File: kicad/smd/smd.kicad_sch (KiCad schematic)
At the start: 13 parts, among them J1 Conn_01x14, J2 Conn_01x14_Socket, J4 Conn_01x03_Socket, J5 Conn_01x06, J6 Conn_01x08, J7 Conn_01x07, J8 Conn_01x09

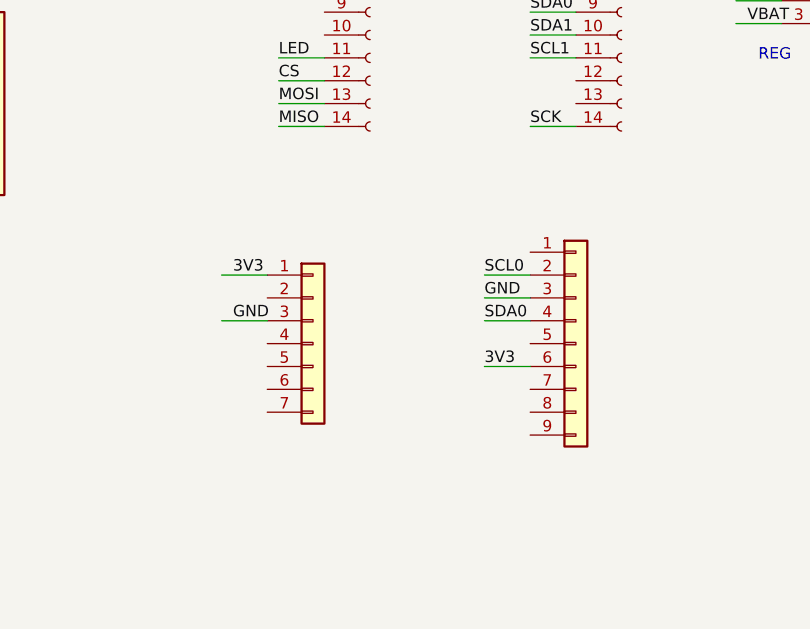
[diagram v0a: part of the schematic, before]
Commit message: modified:   kicad/smd/smd.kicad_pcb
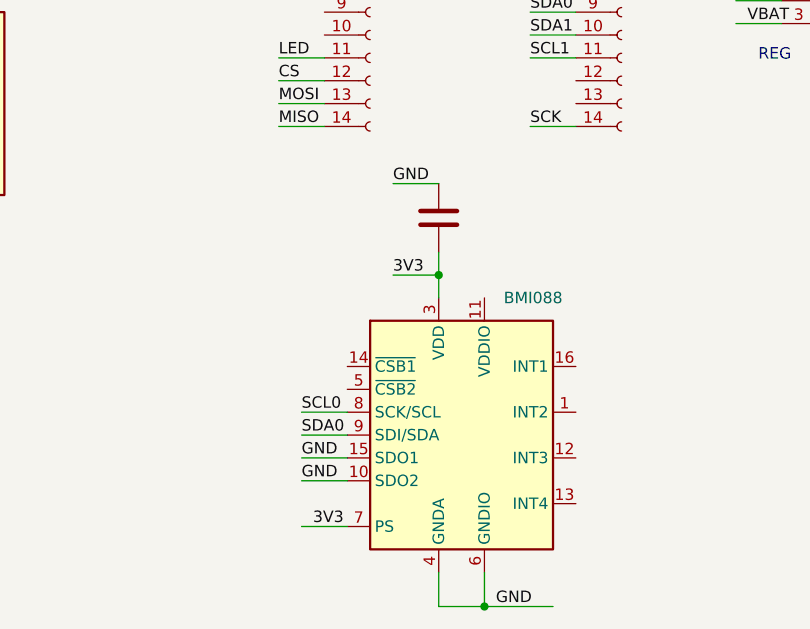
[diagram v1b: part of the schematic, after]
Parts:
- removed J7: Conn_01x07, Connector_PinHeader_1.27mm:PinHeader_1x07_P1.27mm_Vertical, symbol Connector_Generic:Conn_01x07
- removed J8: Conn_01x09, Connector_PinHeader_1.27mm:PinHeader_1x09_P1.27mm_Vertical, symbol Connector_Generic:Conn_01x09
- added C1: C, Capacitor_SMD:C_0603_1608Metric, symbol Device:C
- added U1: BMI088, Package_LGA:Bosch_LGA-16_4.5x3mm_P0.5mm_LayoutBorder7x1y_ClockwisePinNumbering, symbol Sensor_Motion:BMI088
- D1: footprint LED_THT:LED_D3.0mm_FlatTop -> LED_SMD:LED_0603_1608Metric
- R1: footprint Resistor_THT:R_Axial_DIN0204_L3.6mm_D1.6mm_P7.62mm_Horizontal -> Resistor_SMD:R_0603_1608Metric
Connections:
- net 3V3: now also C1.2, U1.3 (VDD), U1.7 (PS)
- net GND: now also C1.1, U1.10 (SDO2), U1.15 (SDO1), U1.2 (GNDA), U1.4 (GNDA), U1.6 (GNDIO)
- net SCL0: now also U1.8 (SCK/SCL)
- net SDA0: now also U1.9 (SDI/SDA)
